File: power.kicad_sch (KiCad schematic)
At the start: 30 parts, among them J2 USB_C_Receptacle_USB2.0, Q1 BC807, U10 LM397, U4 XC6220B331MR, U6 SRV05-4

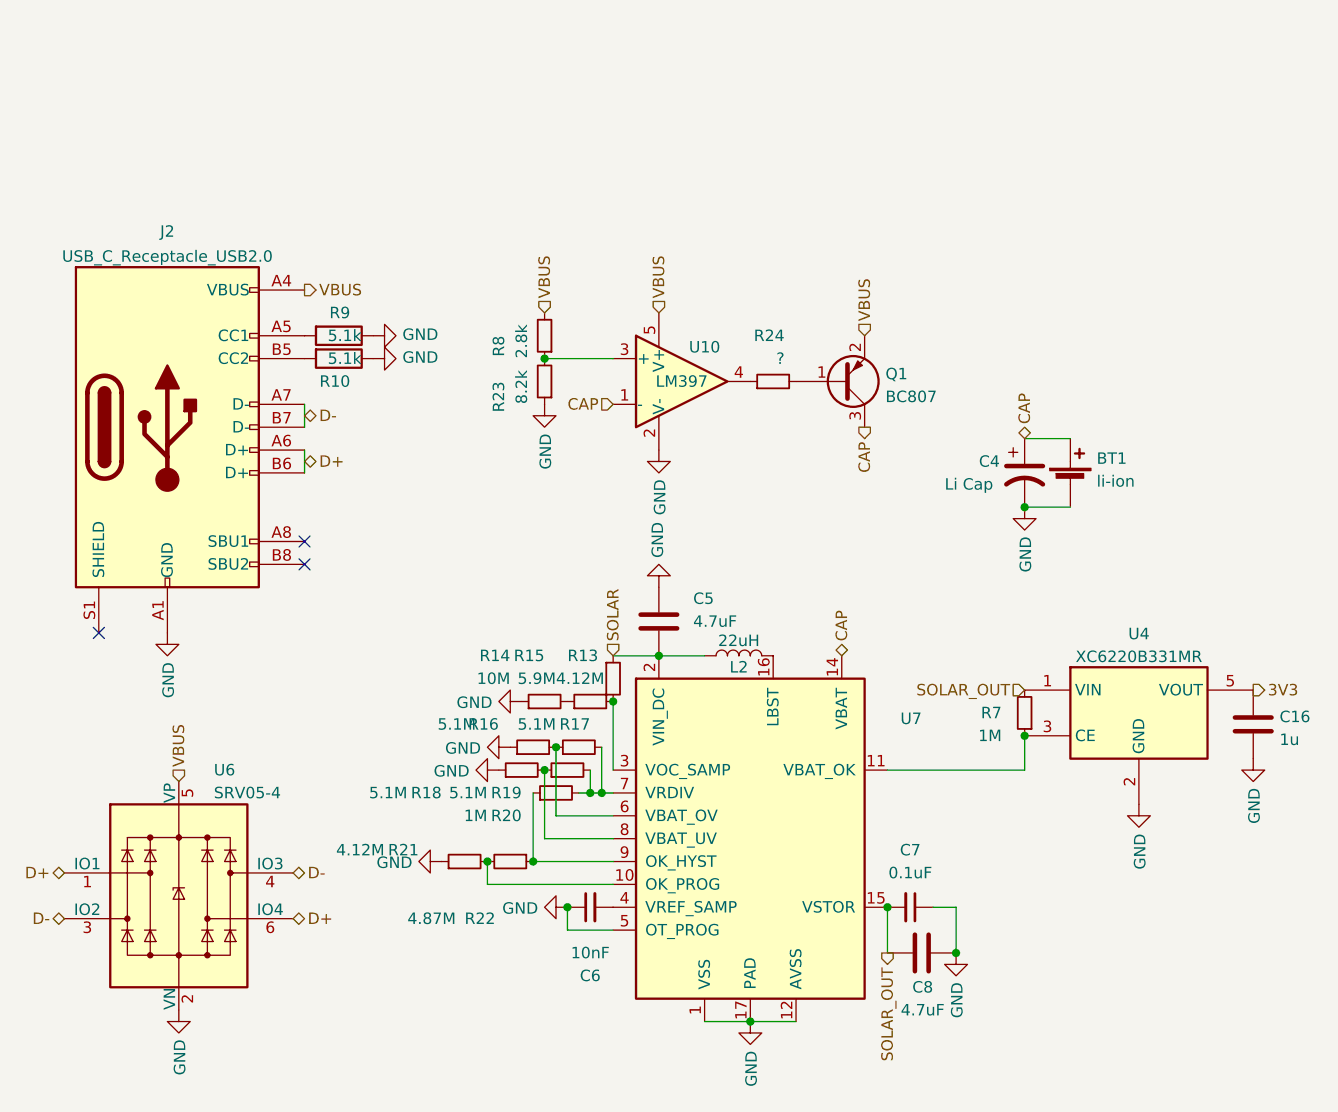
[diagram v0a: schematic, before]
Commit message: swap bms and reg
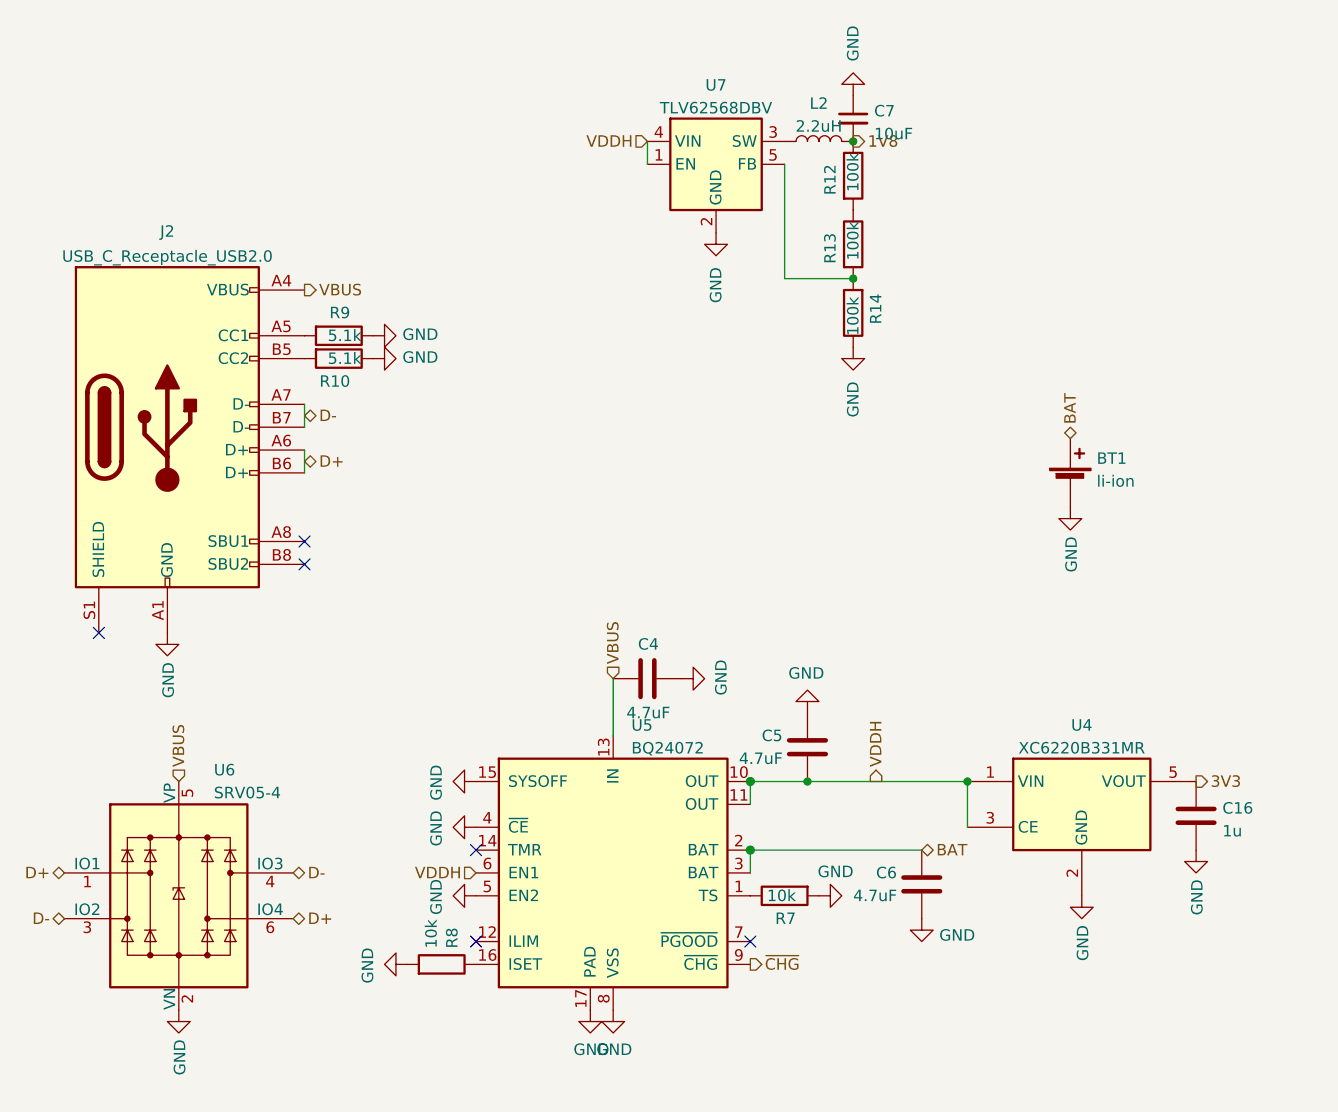
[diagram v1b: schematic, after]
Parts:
- removed C4: Li Cap, Capacitor_THT:CP_Radial_D16.0mm_P7.50mm, symbol Device:C_Polarized_US
- removed C6: 10nF, Capacitor_SMD:C_0603_1608Metric, symbol Device:C_Small
- removed C8: 4.7uF, Capacitor_SMD:C_0805_2012Metric, symbol Device:C
- removed Q1: BC807, Package_TO_SOT_SMD:SOT-23, symbol Transistor_BJT:BC807
- removed R13, R21: 4.12M, Resistor_SMD:R_0603_1608Metric, symbol Device:R_Small
- removed R14: 10M, Resistor_SMD:R_0603_1608Metric, symbol Device:R_Small
- removed R15: 5.9M, Resistor_SMD:R_0603_1608Metric, symbol Device:R_Small
- removed R16, R17, R18, R19: 5.1M, Resistor_SMD:R_0603_1608Metric, symbol Device:R_Small
- removed R20, R7: 1M, Resistor_SMD:R_0603_1608Metric, symbol Device:R_Small
- removed R22: 4.87M, Resistor_SMD:R_0603_1608Metric, symbol Device:R_Small
- removed R23: 8.2k, Resistor_SMD:R_0603_1608Metric, symbol Device:R_Small
- removed R24: ?, Resistor_SMD:R_0603_1608Metric, symbol Device:R_Small
- removed R8: 2.8k, Resistor_SMD:R_0603_1608Metric, symbol Device:R_Small
- removed U10: LM397, Package_TO_SOT_SMD:SOT-23-5, symbol Comparator:LM397
- removed U7: ~, Package_DFN_QFN:QFN-16-1EP_3x3mm_P0.5mm_EP1.7x1.7mm, symbol Battery_Management:BQ25504
- added C4, C6: 4.7uF, Capacitor_SMD:C_0603_1608Metric, symbol Device:C
- added R12, R13, R14: 100k, Resistor_SMD:R_0603_1608Metric, symbol Device:R
- added R7, R8: 10k, Resistor_SMD:R_0603_1608Metric, symbol Device:R
- added U5: BQ24072, Package_DFN_QFN:VQFN-16-1EP_3x3mm_P0.5mm_EP1.68x1.68mm_ThermalVias, symbol Battery_Management:BQ24075
- added U7: TLV62568DBV, Package_TO_SOT_SMD:SOT-23-5, symbol Regulator_Switching:TLV62568DBV
- C7: value 0.1uF -> 10uF
- L2: value 22uH -> 2.2uH; footprint Inductor_SMD:L_Wuerth_WE-TPC-3816 -> Inductor_SMD:L_1008_2520Metric; lcsc-part (none) -> C354533
- U4: lcsc-part (none) -> C5446
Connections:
- net GND: now also C4.2, C6.2, R14.1, R7.2, R8.2, U5.15 (SYSOFF), U5.17 (PAD), U5.4 (~{CE}), U5.5 (EN2), U5.8 (VSS), U7.2 (GND)
- net VBUS: now also C4.1, U5.13 (IN)
- net VDDH: now reaches U4.3 (CE)
- net VDDH: now also C5.2, U4.1 (VIN), U5.10 (OUT), U5.11 (OUT), U5.6 (EN1), U7.1 (EN), U7.4 (VIN)
- net 1V8: now reaches L2.2
- net 1V8: now also C7.2, R12.1
- net CAP renamed BAT
- net BAT: now also C6.1, U5.2 (BAT), U5.3 (BAT)
- net SOLAR: no longer names the net of L2.1
- net SOLAR: now also U7.3 (SW); no longer C5.2
- removed net SOLAR_OUT: C7.2, U4.1 (VIN)
- new net: R12.2, R13.1
- new net: R13.2, R14.2, U7.5 (FB)
- new net: R7.1, U5.1 (TS)
- new net: R8.1, U5.16 (ISET)
- new net ~{CHG}: U5.9 (~{CHG})
- no-connect marks 3 -> 6
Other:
- moved on the sheet: C16, U4
